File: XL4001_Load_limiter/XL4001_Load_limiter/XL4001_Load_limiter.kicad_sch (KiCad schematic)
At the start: 34 parts, among them J1 5.08-2P-90, J2 5.08-2P-90, J3 Conn_01x02_Socket, Q1 PMOS, Q2 2N7002K, U1 XL4001

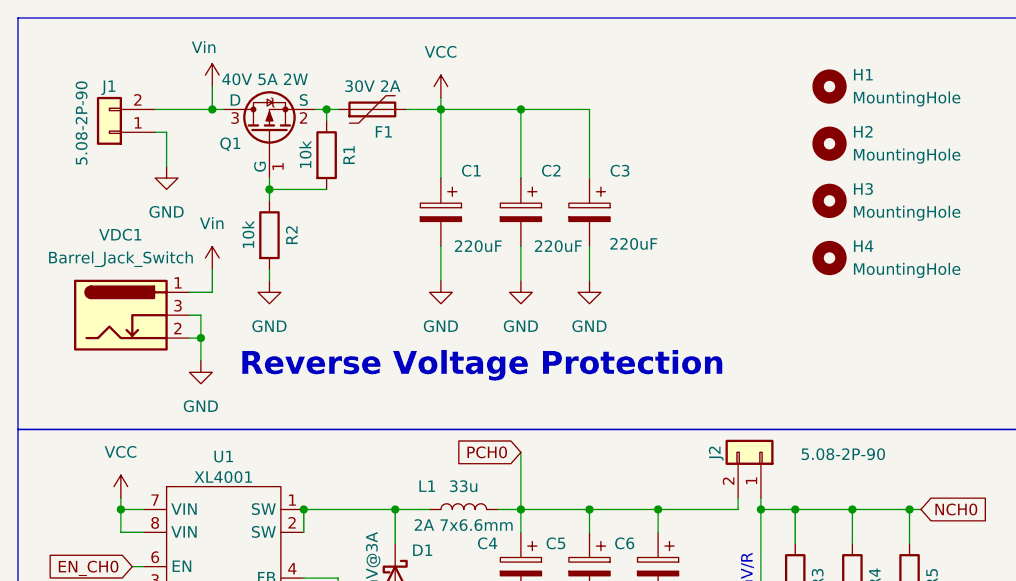
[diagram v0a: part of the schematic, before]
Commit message: Quick sync
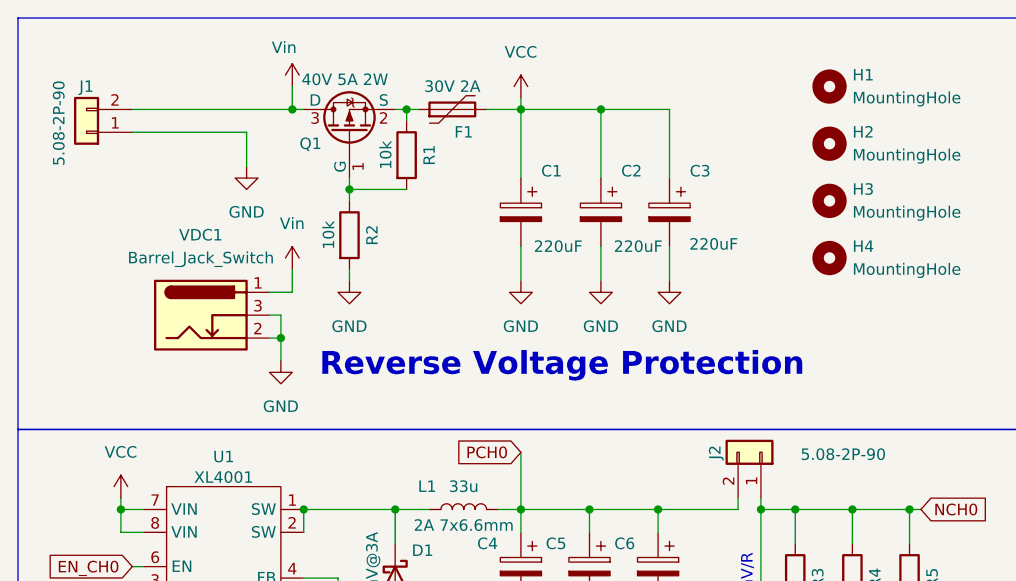
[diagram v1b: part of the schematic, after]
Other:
- moved on the sheet: C1, C2, C3, F1, J1, Q1, R1, R2, VDC1

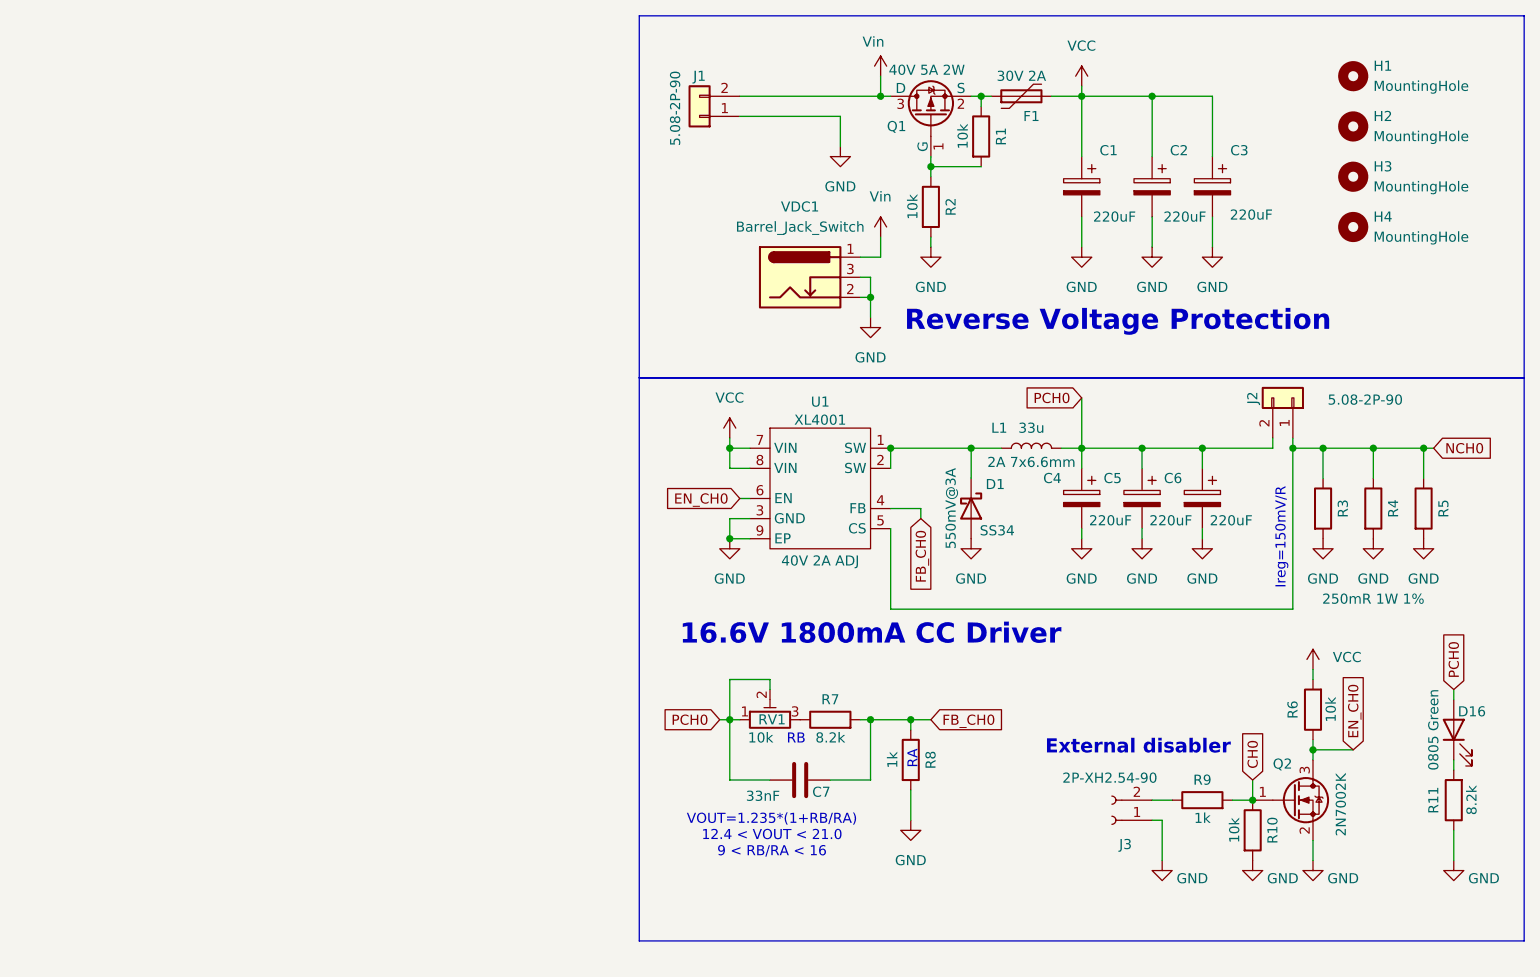
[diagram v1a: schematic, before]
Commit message: Xl4001 update
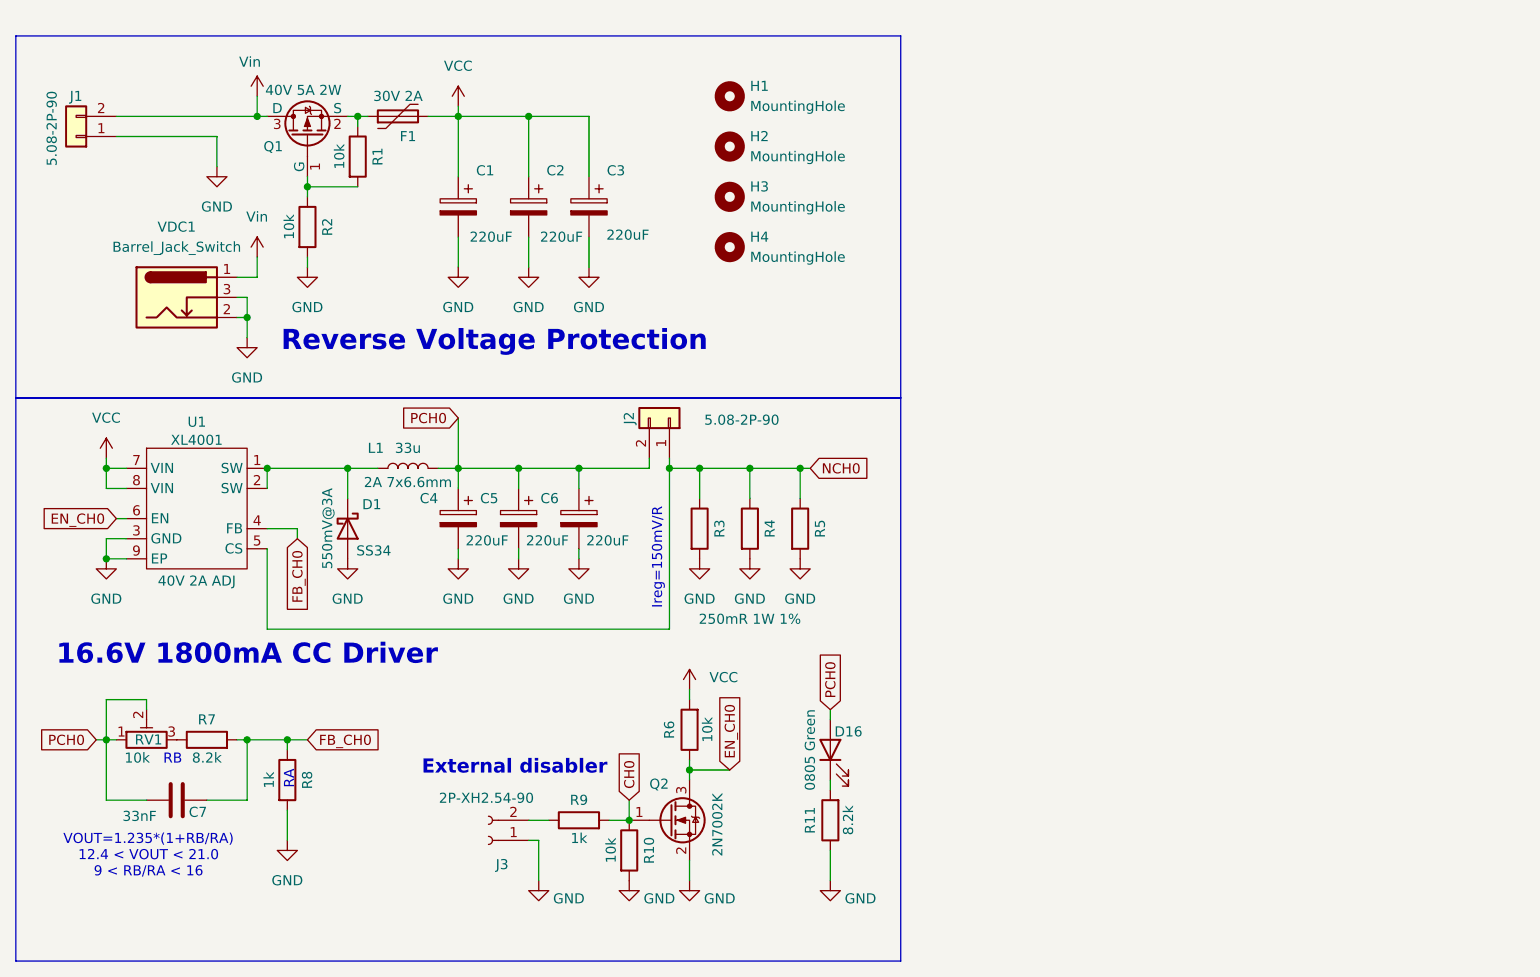
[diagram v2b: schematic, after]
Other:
- title: (none) -> XL4001 Load limiter
- moved on the sheet: C1, C2, C3, C4, C5, C6, C7, D1, D16, F1, H1, H2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

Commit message: Sincronização de arquivos
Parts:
- C1, C2, C3, C4, C5, C6: footprint Capacitor_SMD:CP_Elec_6.3x7.7 -> Aleoexpress:Cap_polymer
